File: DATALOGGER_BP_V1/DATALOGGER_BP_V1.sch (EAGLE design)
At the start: 69 parts, among them IC1 TRV1-1222M, J1 1985247, J2 1985247, J3 1985247, J4 1985247, J5 1985247, J6 1985247, J7 1985247, J8 1985247, J9 1755736, U1 AD620ARZ-REEL7, U2 AD620ARZ-REEL7, U3 AD620ARZ-REEL7, U4 AD620ARZ-REEL7, U5 AD620ARZ-REEL7, U6 AD620ARZ-REEL7, U7 AD620ARZ-REEL7, U8 AD620ARZ-REEL7

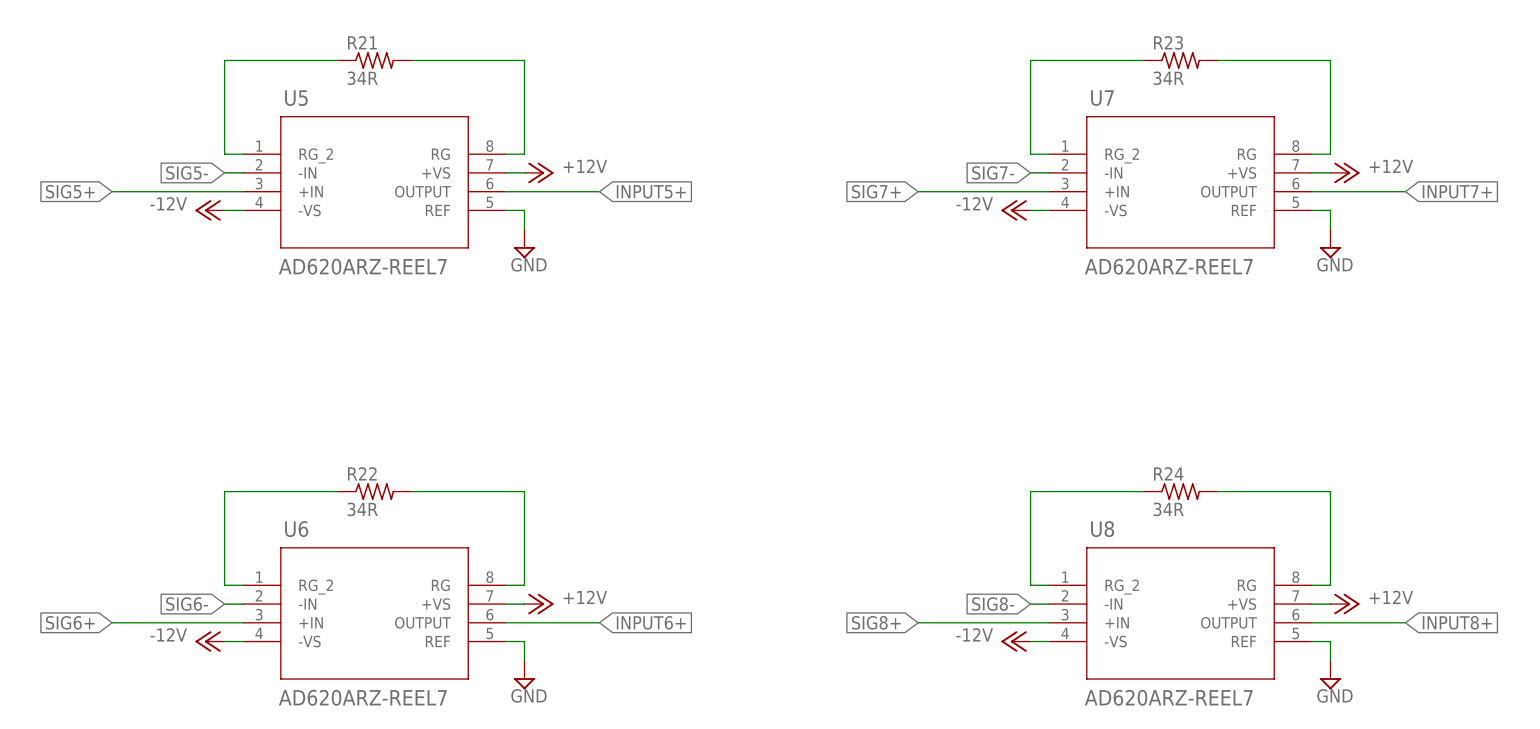
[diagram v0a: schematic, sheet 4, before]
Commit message: tarjeta_v22
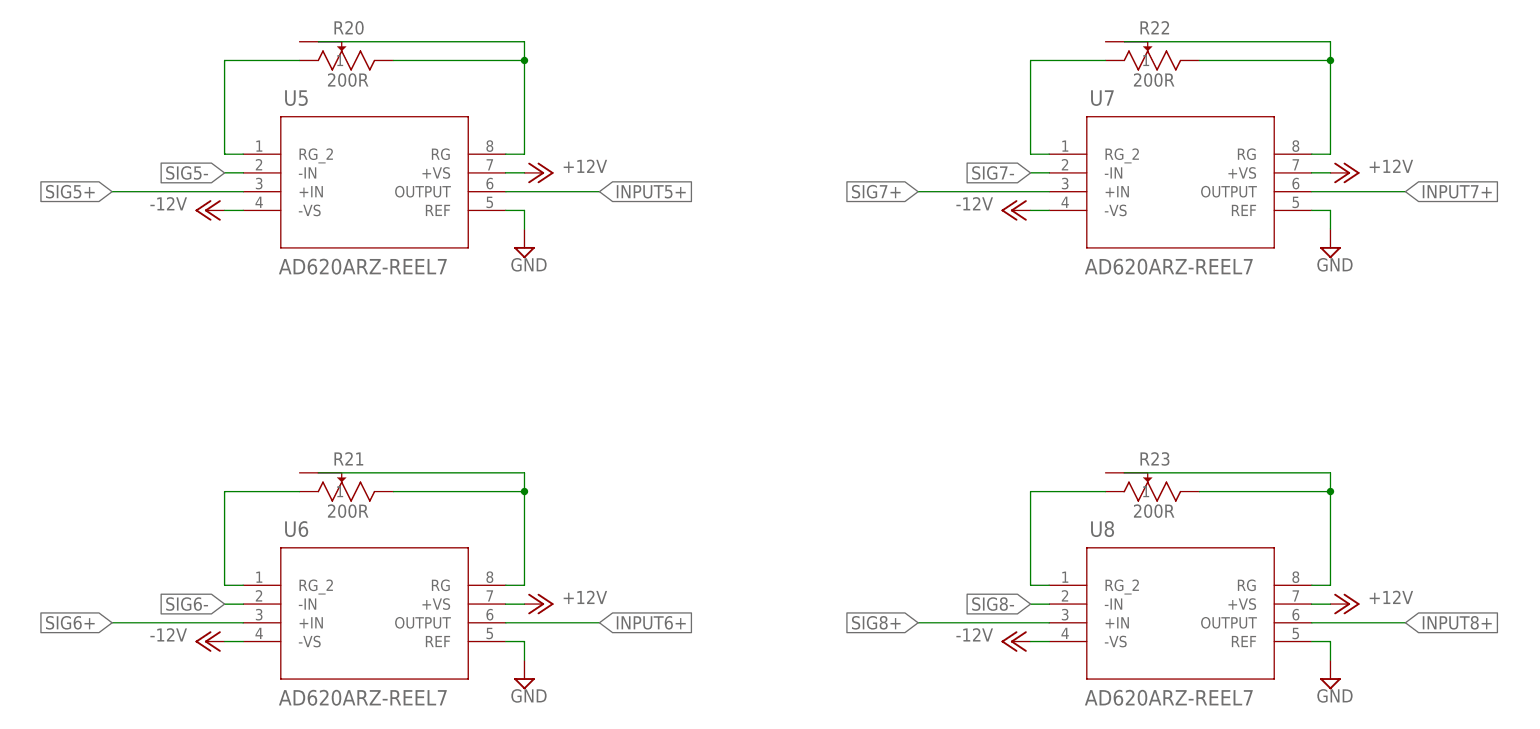
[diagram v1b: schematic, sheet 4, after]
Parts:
- removed R24: 34R, rcl:R-US_R0805
- added R25: 200R, 22AR200LFTR:22AR200LFTR
- R17, R18, R19, R20, R21, R22, R23: value 34R -> 200R; device rcl:R-US_R0805 -> 22AR200LFTR:22AR200LFTR
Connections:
- net N$17: now also R25.1; no longer R17.1
- net N$18: now also R25.2, R25.3; no longer R17.2
- net N$19: now also R17.1; no longer R18.1
- net N$20: now also R17.2, R17.3; no longer R18.2
- net N$21: now also R18.1; no longer R19.1
- net N$22: now also R18.2, R18.3; no longer R19.2
- net N$23: now also R19.1; no longer R20.1
- net N$24: now also R19.2, R19.3; no longer R20.2
- net N$25: now also R20.1; no longer R21.1
- net N$26: now also R20.2, R20.3; no longer R21.2
- net N$27: now also R21.1; no longer R22.1
- net N$28: now also R21.2, R21.3; no longer R22.2
- net N$29: now also R22.1; no longer R23.1
- net N$30: now also R22.2, R22.3; no longer R23.2
- net N$31: now also R23.1; no longer R24.1
- net N$32: now also R23.2, R23.3; no longer R24.2
